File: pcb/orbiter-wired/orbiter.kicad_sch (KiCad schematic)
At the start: 18 parts, among them J1 SWD, J3 I2C Extension, J5 Keyboard matrix, U1 TPS82140SILR

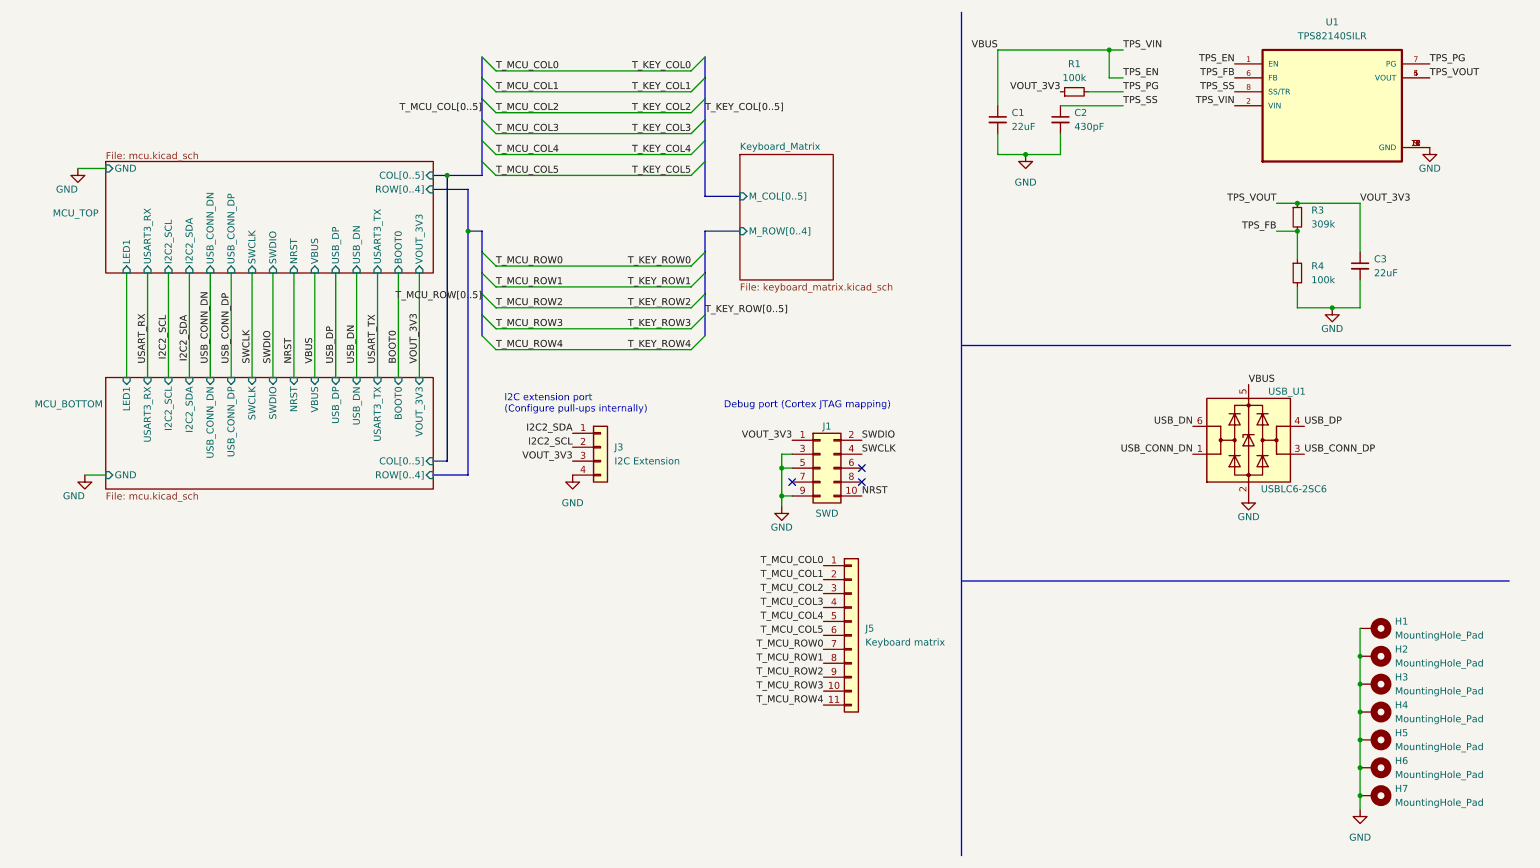
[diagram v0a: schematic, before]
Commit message: Add TODOs for fixes for next version
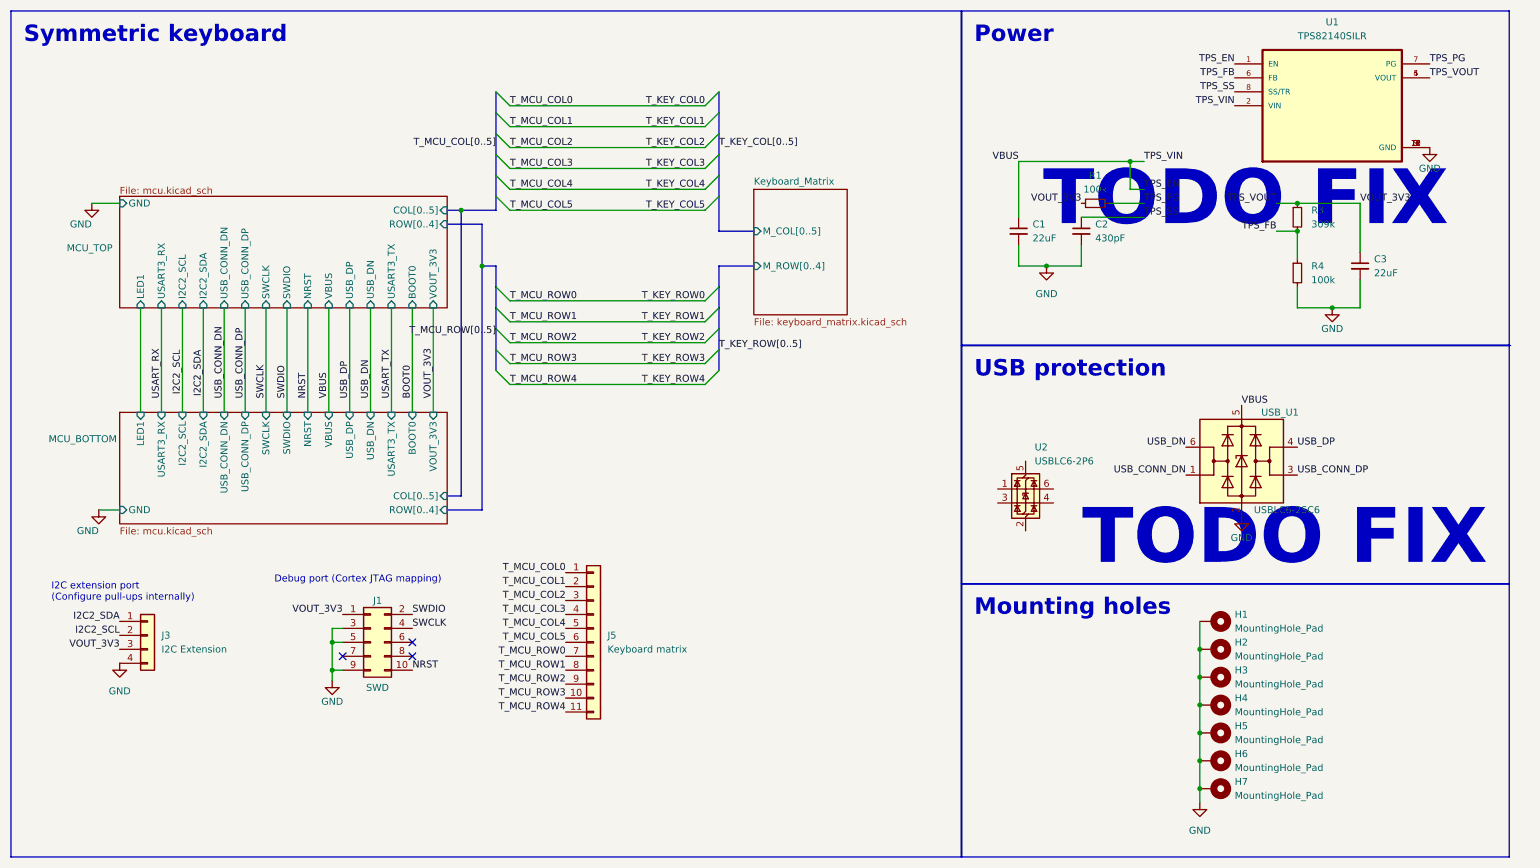
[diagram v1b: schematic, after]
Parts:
- added U2: USBLC6-2P6, Package_TO_SOT_SMD:SOT-666, symbol Power_Protection:USBLC6-2P6
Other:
- note added: "TODO FIX"
- moved on the sheet: C1, C2, H1, H2, H3, H4, H5, H6, H7, J1, J3, J5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
